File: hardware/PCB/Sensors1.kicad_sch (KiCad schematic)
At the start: 44 parts, among them J201 ina333, J202 ACS712, J203 BMP3, U201 INA333xxDGK, U202 MCP6002T-I/SN, U203 TLV431, U204 QNHC3, U205 TLV431, U206 ACS712xLCTR-05B

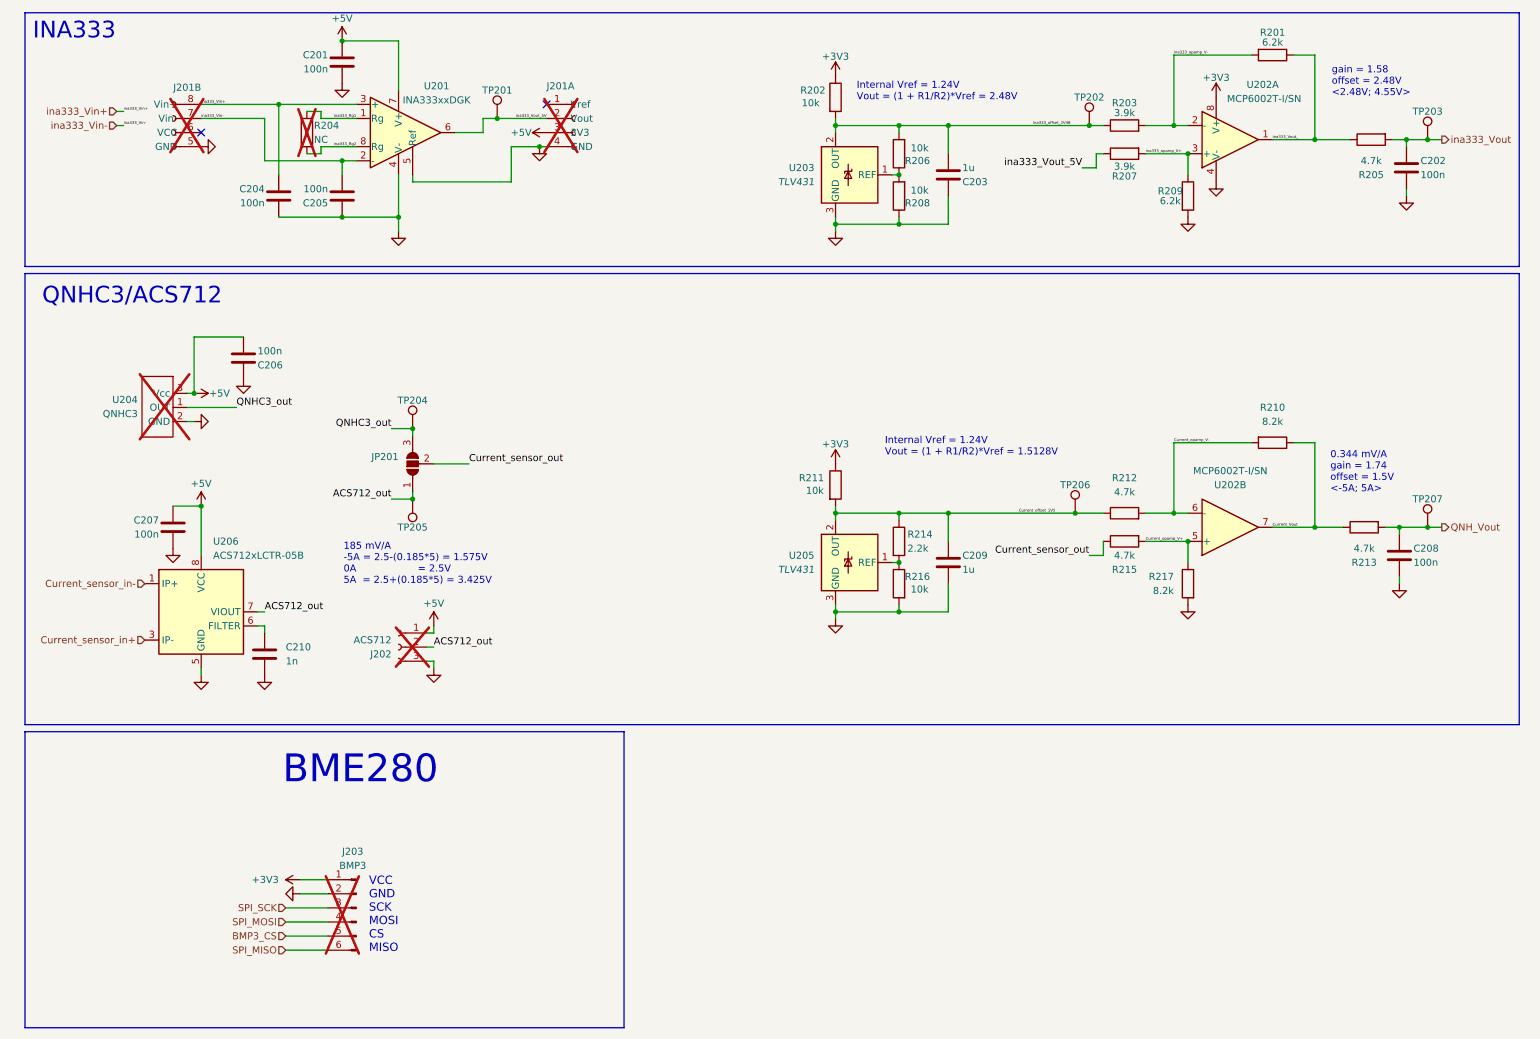
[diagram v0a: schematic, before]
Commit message: usb, sd
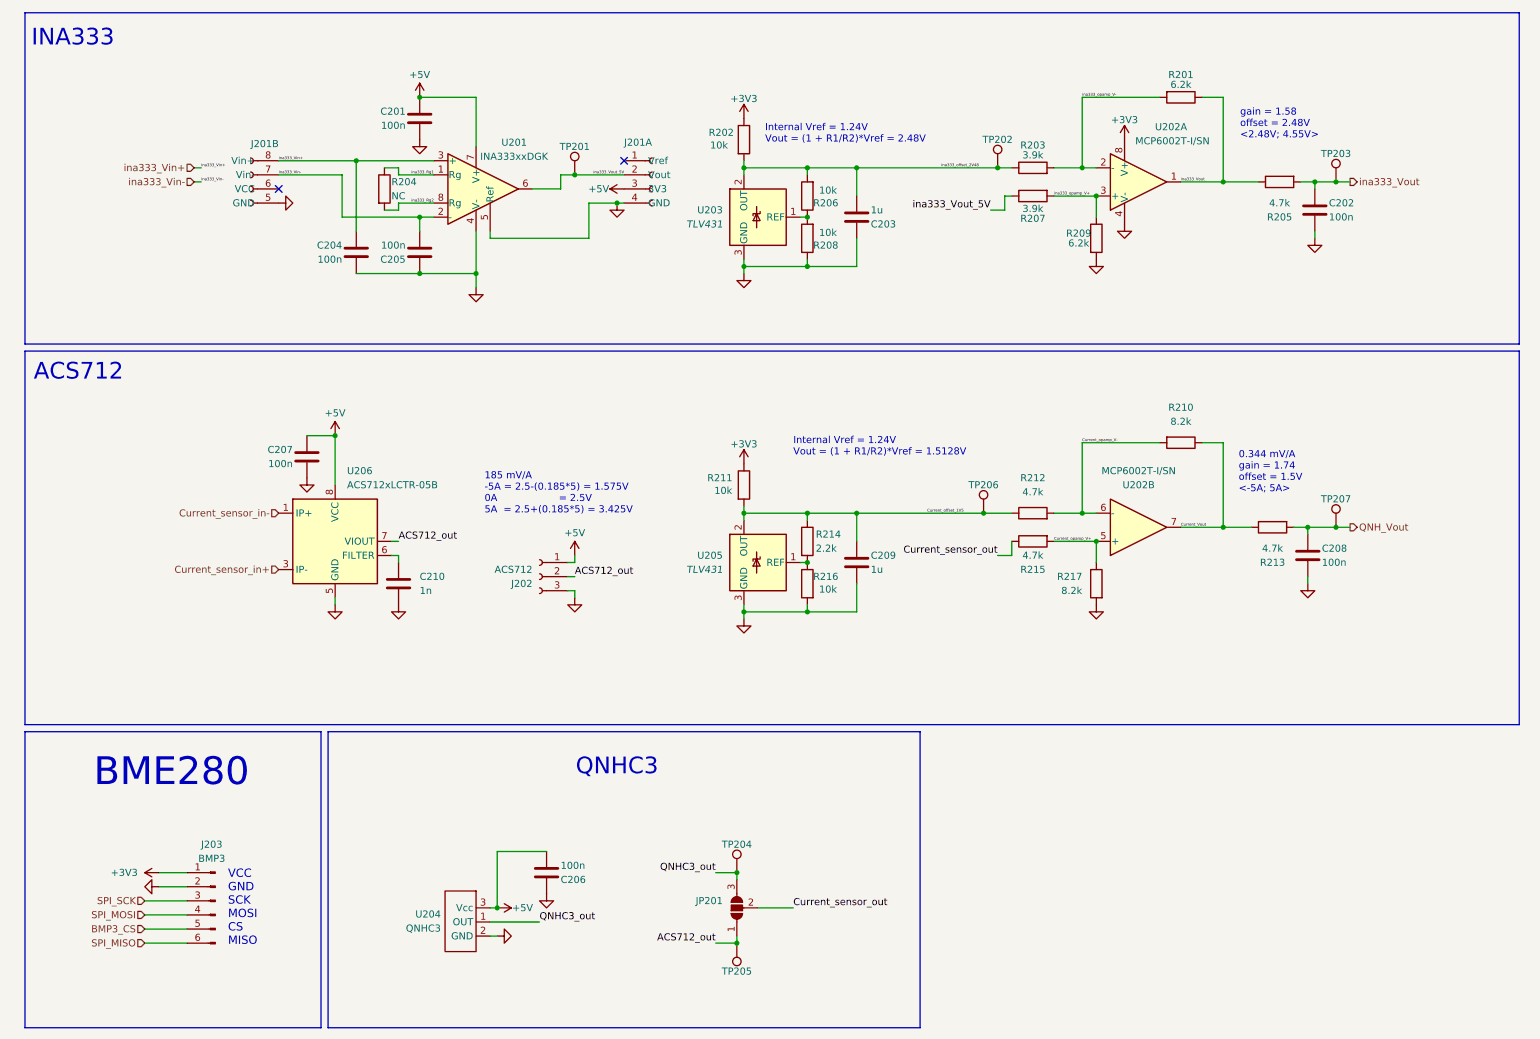
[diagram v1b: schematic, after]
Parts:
- J201, J202, J203, R204, U204: now fitted
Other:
- note added: "ACS712"
- note added: "QNHC3"
- note removed: "QNHC3/ACS712"
- title: (none) -> Stanowisko do badania parametrów pracy ogniw Li-Ion Li-Pol
- moved on the sheet: C201, C202, C203, C204, C205, C206, C207, C208, C209, C210, JP201, R201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
